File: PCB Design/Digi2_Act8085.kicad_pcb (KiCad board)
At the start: 2 copper layers, 27 parts, among them U1 8085A, U10 8255, U2 Barrel_Jack, U3 L7805, U4 2764, U5 CY6264, U6 74LS373, U7 74LS138, U8 8255, U9 8255, Y1 3MHz

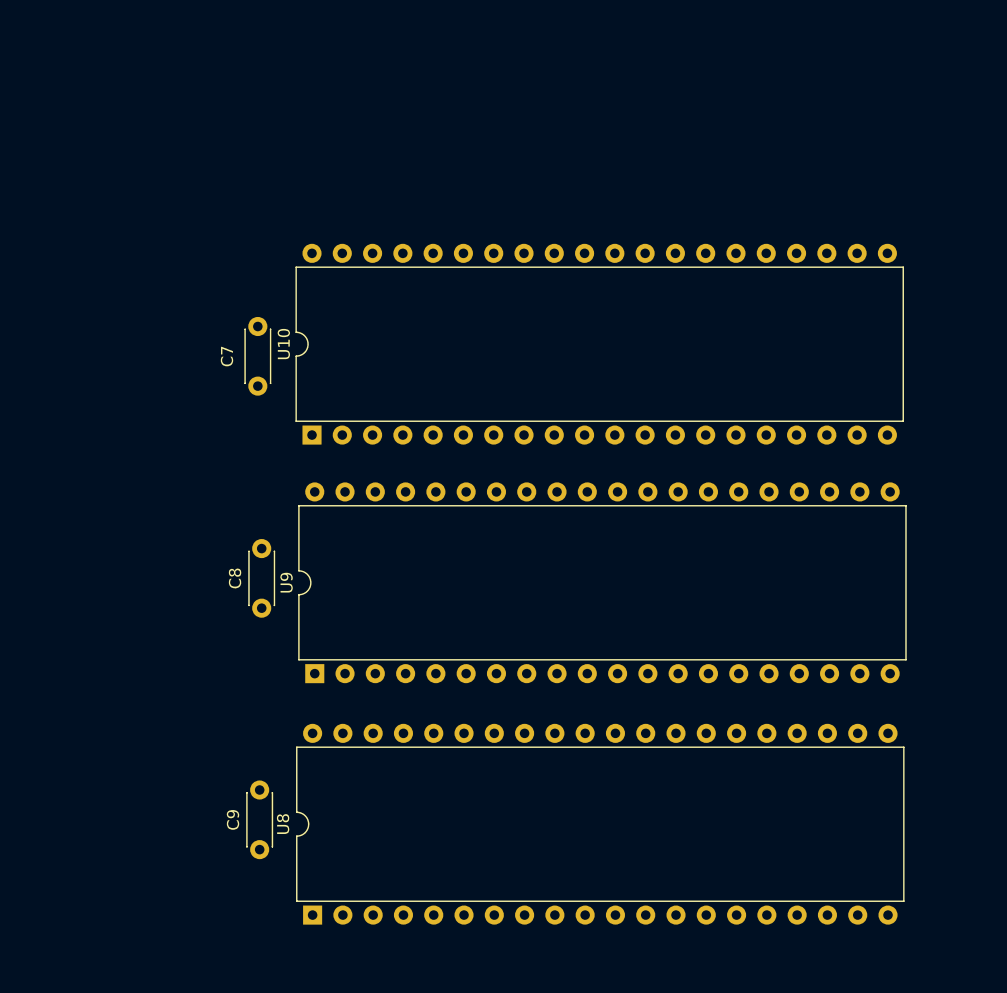
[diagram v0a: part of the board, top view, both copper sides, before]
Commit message: Peripheral Routing
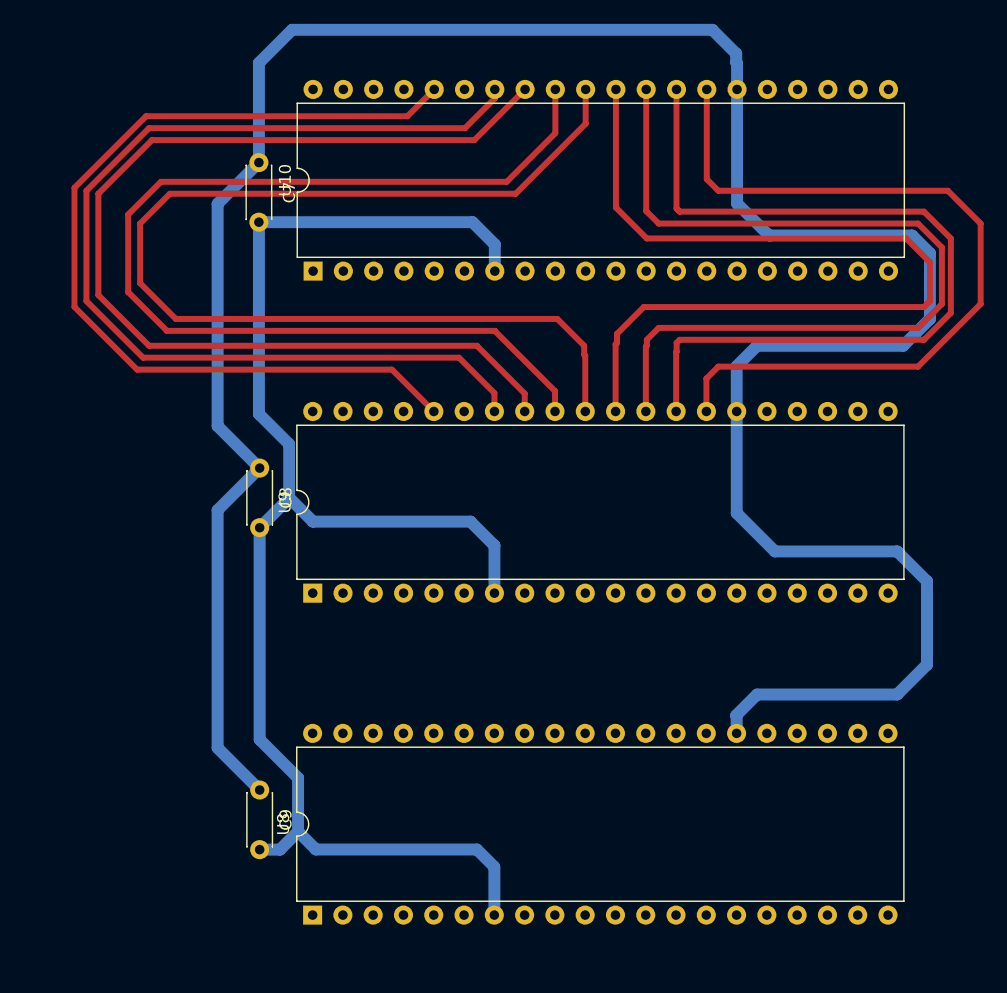
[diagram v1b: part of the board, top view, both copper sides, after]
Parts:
- moved C7 18.8 mm to (156.5, 33.9), turned to -90 degrees
- moved U10 13.8 mm to (161.0, 43.0)
- moved C8 11.8 mm to (156.5, 59.5), turned to -90 degrees
- moved U9 6.75 mm to (161.0, 70.0)
- moved C9 5.00 mm to (156.5, 86.5), turned to -90 degrees
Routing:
- net +5V: track 68.5 -> 288.2 mm
- net GND: track 69.4 -> 195.2 mm
- net /Memory and Peripheral Inteface/AD3: track 50.6 -> 144.3 mm
- net /Memory and Peripheral Inteface/AD2: track 52.8 -> 142.5 mm
- net /Memory and Peripheral Inteface/AD1: track 60.7 -> 149.2 mm
- net /Memory and Peripheral Inteface/AD0: track 62.5 -> 148.9 mm
- net /Memory and Peripheral Inteface/~{WR}: track 0.00 -> 77.4 mm
- net /Memory and Peripheral Inteface/AD4: track 69.9 -> 145.3 mm
- net /Memory and Peripheral Inteface/AD5: track 66.3 -> 139.3 mm
- net /Memory and Peripheral Inteface/AD6: track 69.5 -> 139.6 mm
- net /Memory and Peripheral Inteface/AD7: track 65.5 -> 132.7 mm

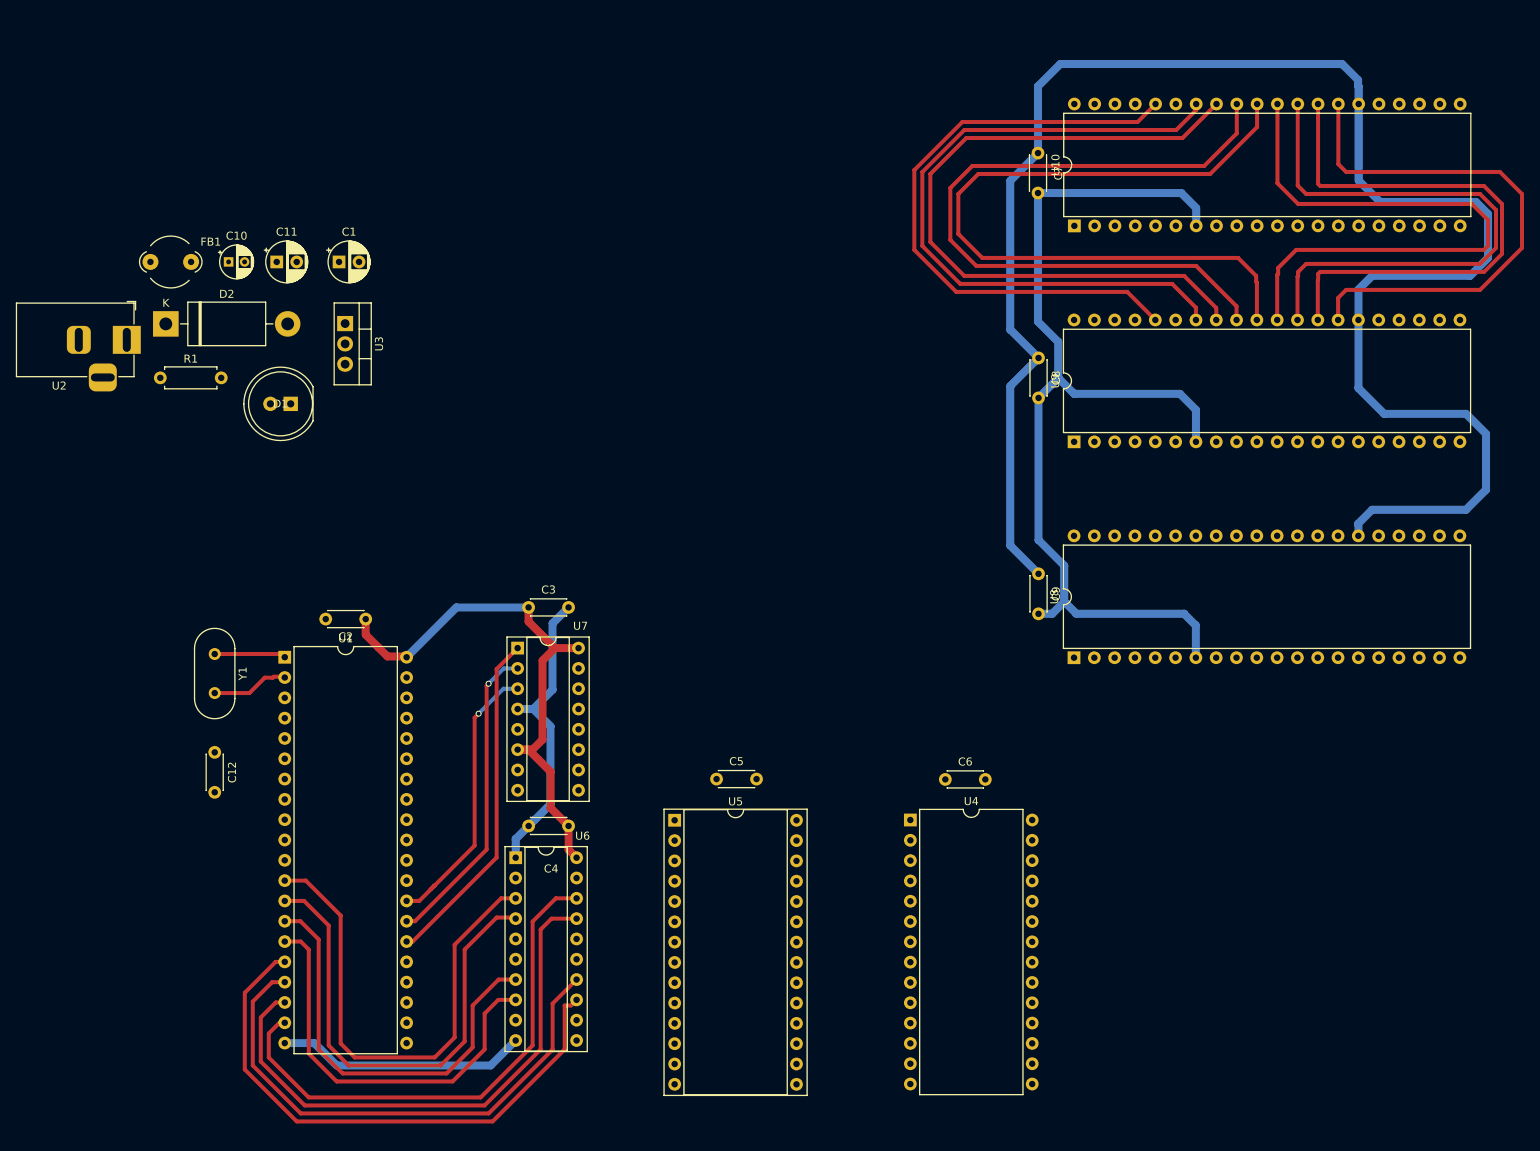
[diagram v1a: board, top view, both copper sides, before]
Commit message: Additional Route
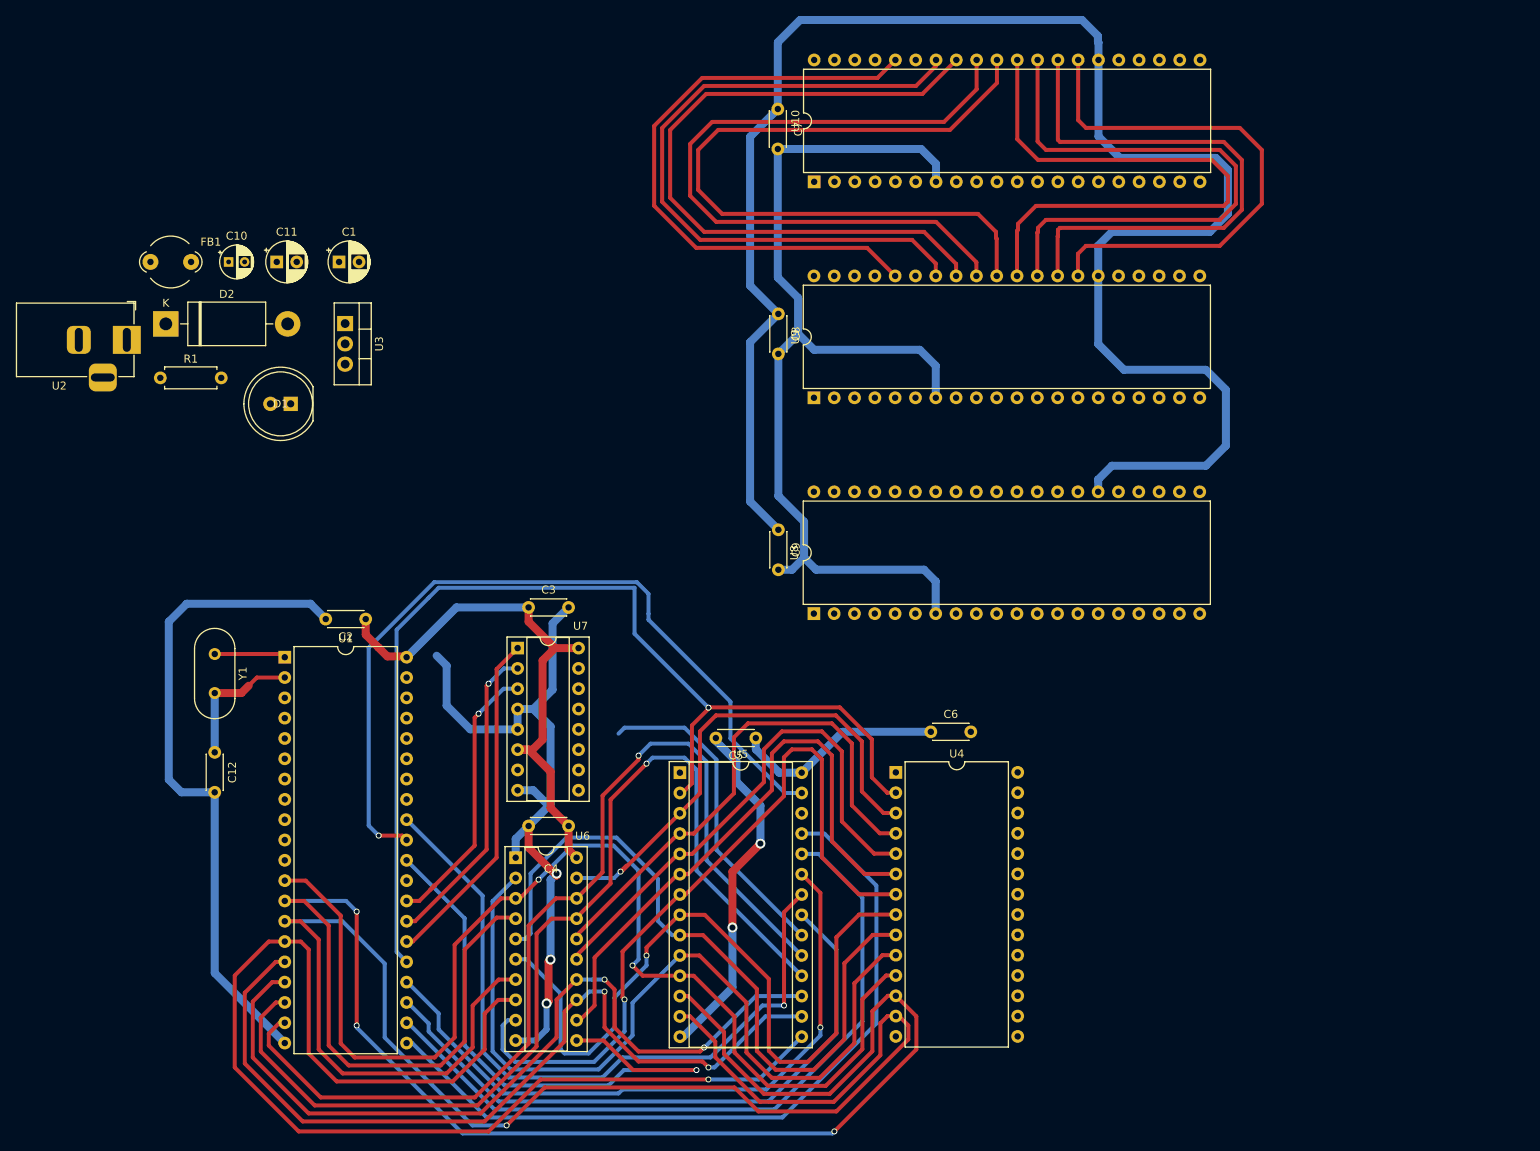
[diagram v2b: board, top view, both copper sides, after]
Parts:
- moved C7 33.0 mm to (123.9, 28.4)
- moved C8 33.0 mm to (124.0, 54.0)
- moved C9 33.0 mm to (124.0, 81.0)
- moved U10 33.0 mm to (128.5, 37.5)
- moved U8 33.0 mm to (128.4, 91.5)
- moved U9 33.0 mm to (128.4, 64.5)
- moved C5 7.11 mm to (121.2, 107.0), turned to 180 degrees
- moved C6 6.23 mm to (143.1, 106.3)
- moved U4 6.23 mm to (138.7, 111.3)
- moved U5 5.99 mm to (111.7, 111.4)
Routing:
- net /Memory and Peripheral Inteface/AD1: track 149.2 -> 302.6 mm, vias 0 -> 3
- net GND: track 195.2 -> 347.7 mm, vias 0 -> 5
- net /Memory and Peripheral Inteface/AD2: track 142.5 -> 287.0 mm, vias 0 -> 1
- net /Memory and Peripheral Inteface/A12: track 0.00 -> 135.9 mm, vias 0 -> 1
- net /Memory and Peripheral Inteface/A0: track 0.00 -> 103.3 mm
- net /Memory and Peripheral Inteface/~{WR}: track 77.4 -> 178.2 mm, vias 0 -> 1
- net /Memory and Peripheral Inteface/AD3: track 144.3 -> 243.2 mm, vias 0 -> 1
- net /Memory and Peripheral Inteface/A8: track 0.00 -> 96.8 mm
- net /Memory and Peripheral Inteface/A2: track 0.00 -> 94.8 mm, vias 0 -> 1
- net /Memory and Peripheral Inteface/A3: track 0.00 -> 94.7 mm, vias 0 -> 1
- net /Memory and Peripheral Inteface/A9: track 0.00 -> 91.4 mm
- net /Memory and Peripheral Inteface/~{RD}: track 0.00 -> 90.5 mm, vias 0 -> 1
- net /Memory and Peripheral Inteface/A1: track 0.00 -> 89.4 mm
- net /Memory and Peripheral Inteface/A11: track 0.00 -> 82.8 mm, vias 0 -> 1
- net /Memory and Peripheral Inteface/AD0: track 148.9 -> 231.6 mm, vias 0 -> 2
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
